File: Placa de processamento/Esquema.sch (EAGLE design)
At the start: 11 parts

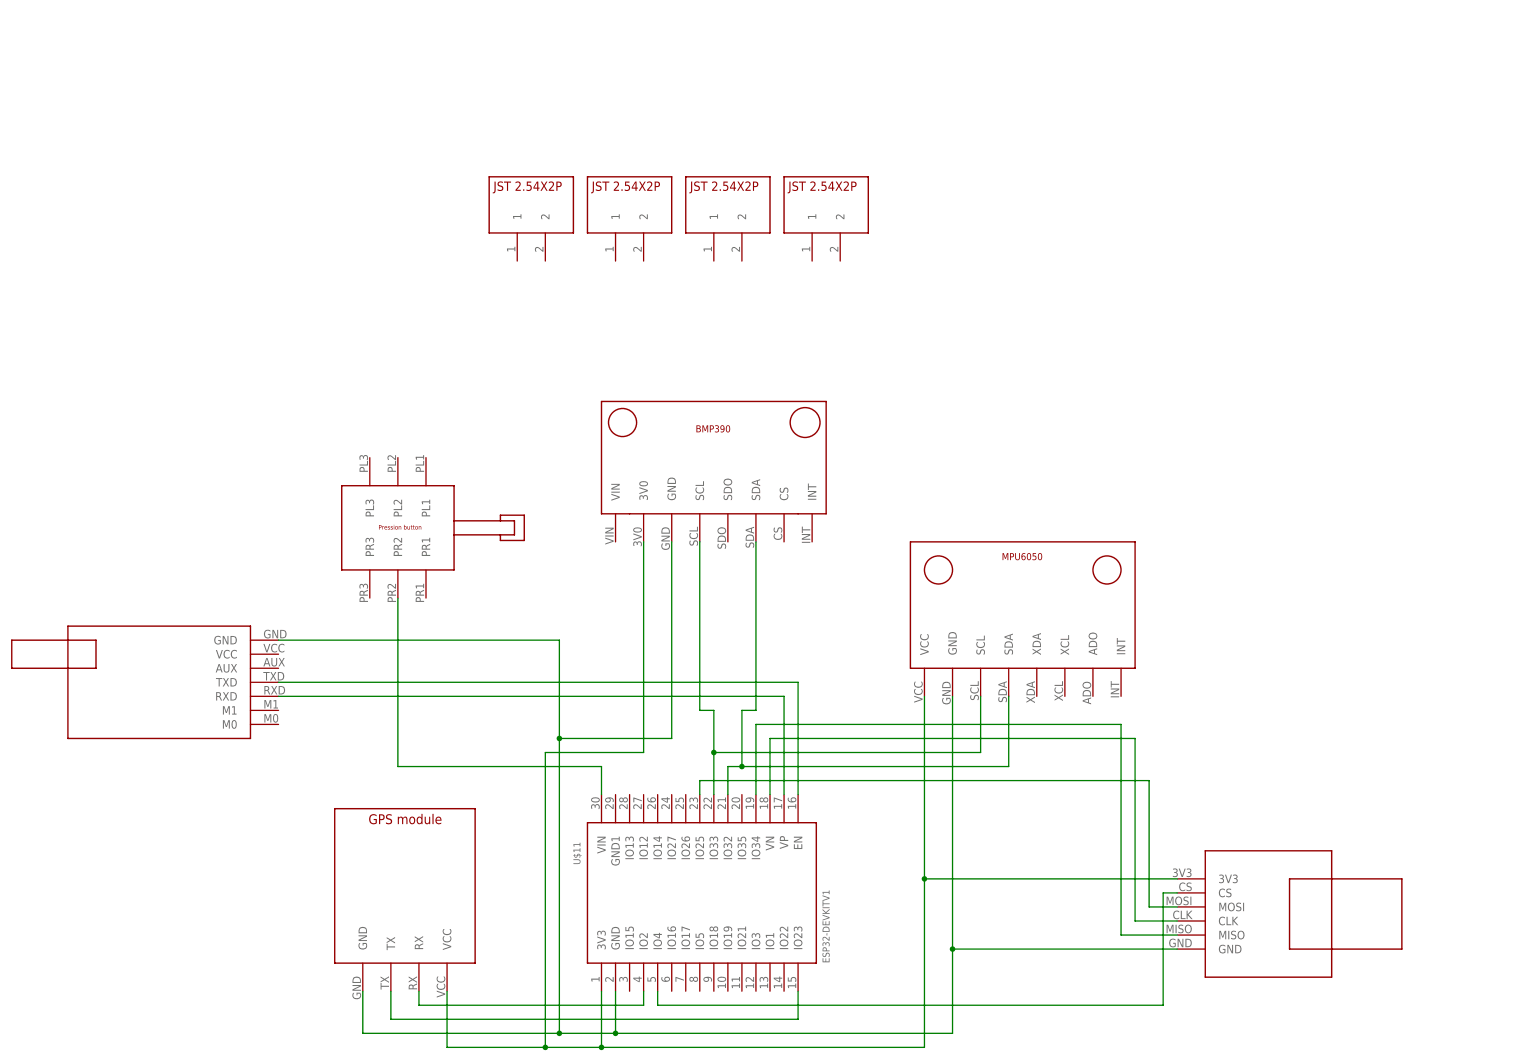
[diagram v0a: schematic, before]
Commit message: Roteamento da placa
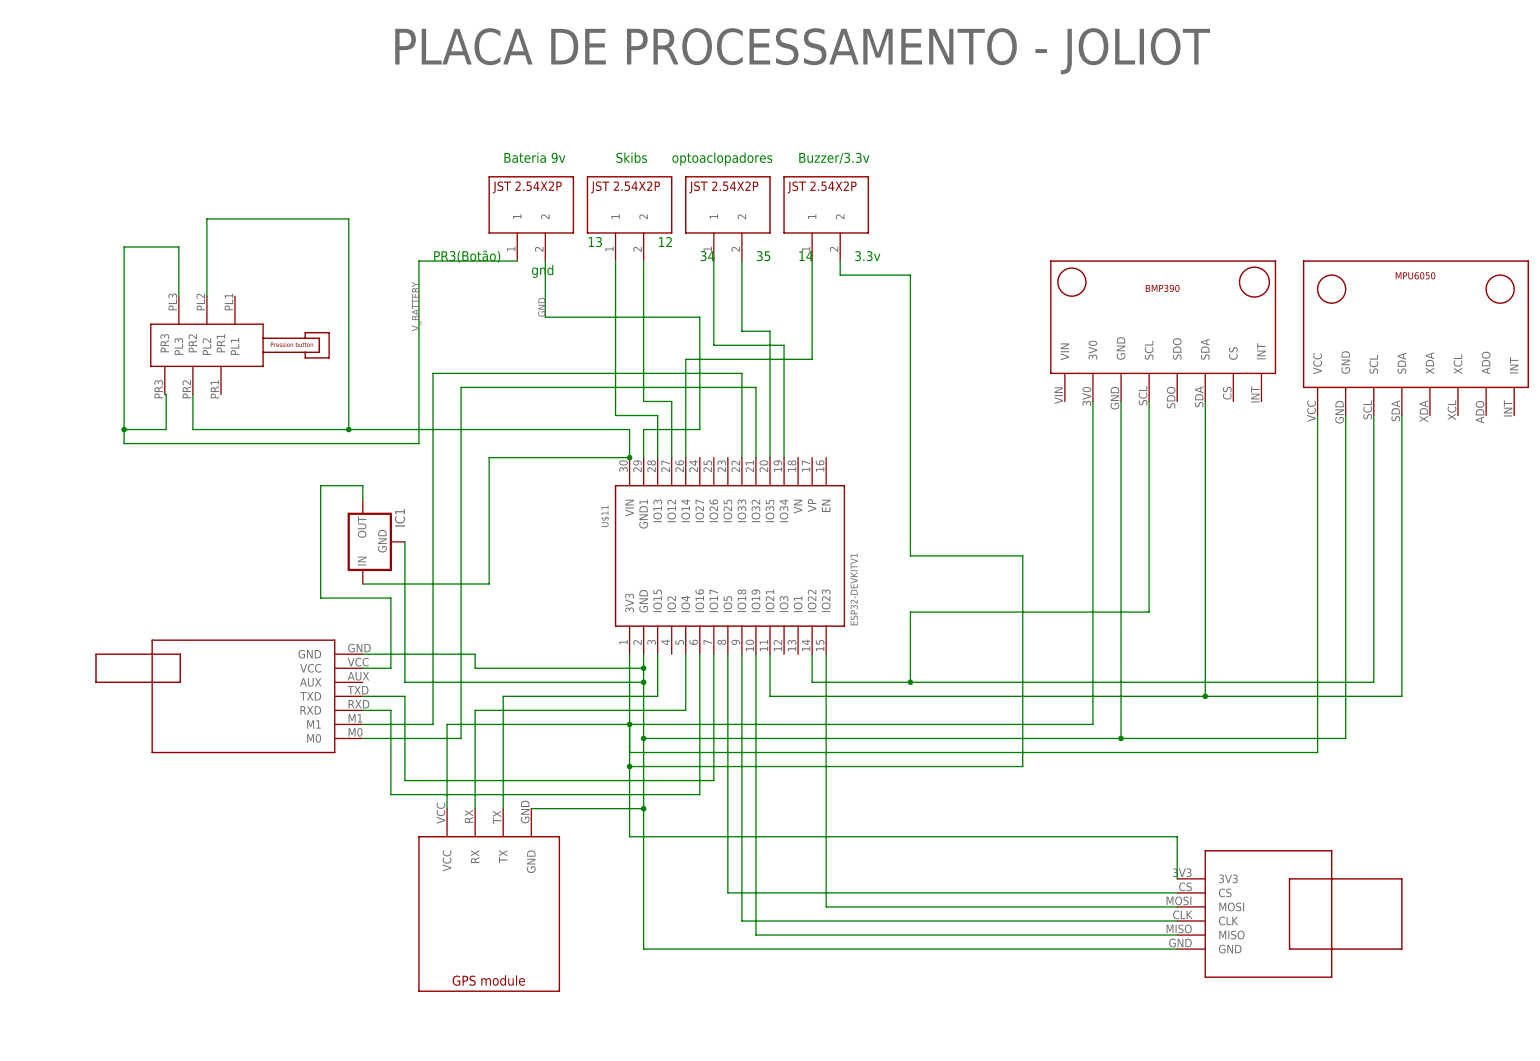
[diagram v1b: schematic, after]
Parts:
- added IC1: (no value), v-reg:78LXX
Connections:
- new net GND: U$11.GND1, U$7.2
- new net N$12: IC1.OUT, U$2.VCC
- new net N$15: U$11.IO18, U$8.CLK
- new net N$16: U$11.IO19, U$8.MISO
- new net N$19: U$11.IO13, U$6.1
- new net N$20: U$11.IO12, U$6.2
- new net N$21: U$11.IO14, U$4.1
- new net N$22: U$11.IO34, U$5.1
- new net N$23: U$11.IO35, U$5.2
- new net V_BATTERY: U$10.PL3, U$10.PR3, U$7.1
- net N$1: now also U$11.IO21; no longer U$11.IO32
- net N$10: now also U$11.IO33, U$2.M1; no longer U$11.IO34, U$8.MISO
- net N$11: now also U$11.IO32, U$2.M0; no longer U$10.PR2, U$11.VIN
- net N$13: now also U$11.IO5, U$8.CS; no longer U$11.VP, U$2.RXD
- net N$14: now also U$11.IO23, U$8.MOSI; no longer U$11.EN, U$2.TXD
- net N$2: now also U$11.IO22; no longer U$11.IO33
- net N$3: now also U$4.2
- net N$4: now also IC1.GND
- net N$5: now also U$11.IO4, U$3.RX; no longer U$11.IO23, U$3.TX
- net N$6: now also U$11.IO15, U$3.TX; no longer U$11.IO2, U$3.RX
- net N$7: now also IC1.IN, U$10.PL2, U$10.PR2, U$11.VIN; no longer U$11.IO4, U$8.CS
- net N$8: now also U$11.IO17, U$2.TXD; no longer U$11.IO25, U$8.MOSI
- net N$9: now also U$11.IO16, U$2.RXD; no longer U$11.VN, U$8.CLK
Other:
- note added: "12"
- note added: "13"
- note added: "14"
- note added: "3.3v"
- note added: "34"
- note added: "35"
- note added: "Bateria 9v"
- note added: "Buzzer/3.3v"
- note added: "PLACA DE PROCESSAMENTO - JOLIOT"
- note added: "PR3(Botão)"
- note added: "Skibs"
- note added: "gnd"
- note added: "optoaclopadores"
- moved on the sheet: U$11

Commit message: Update
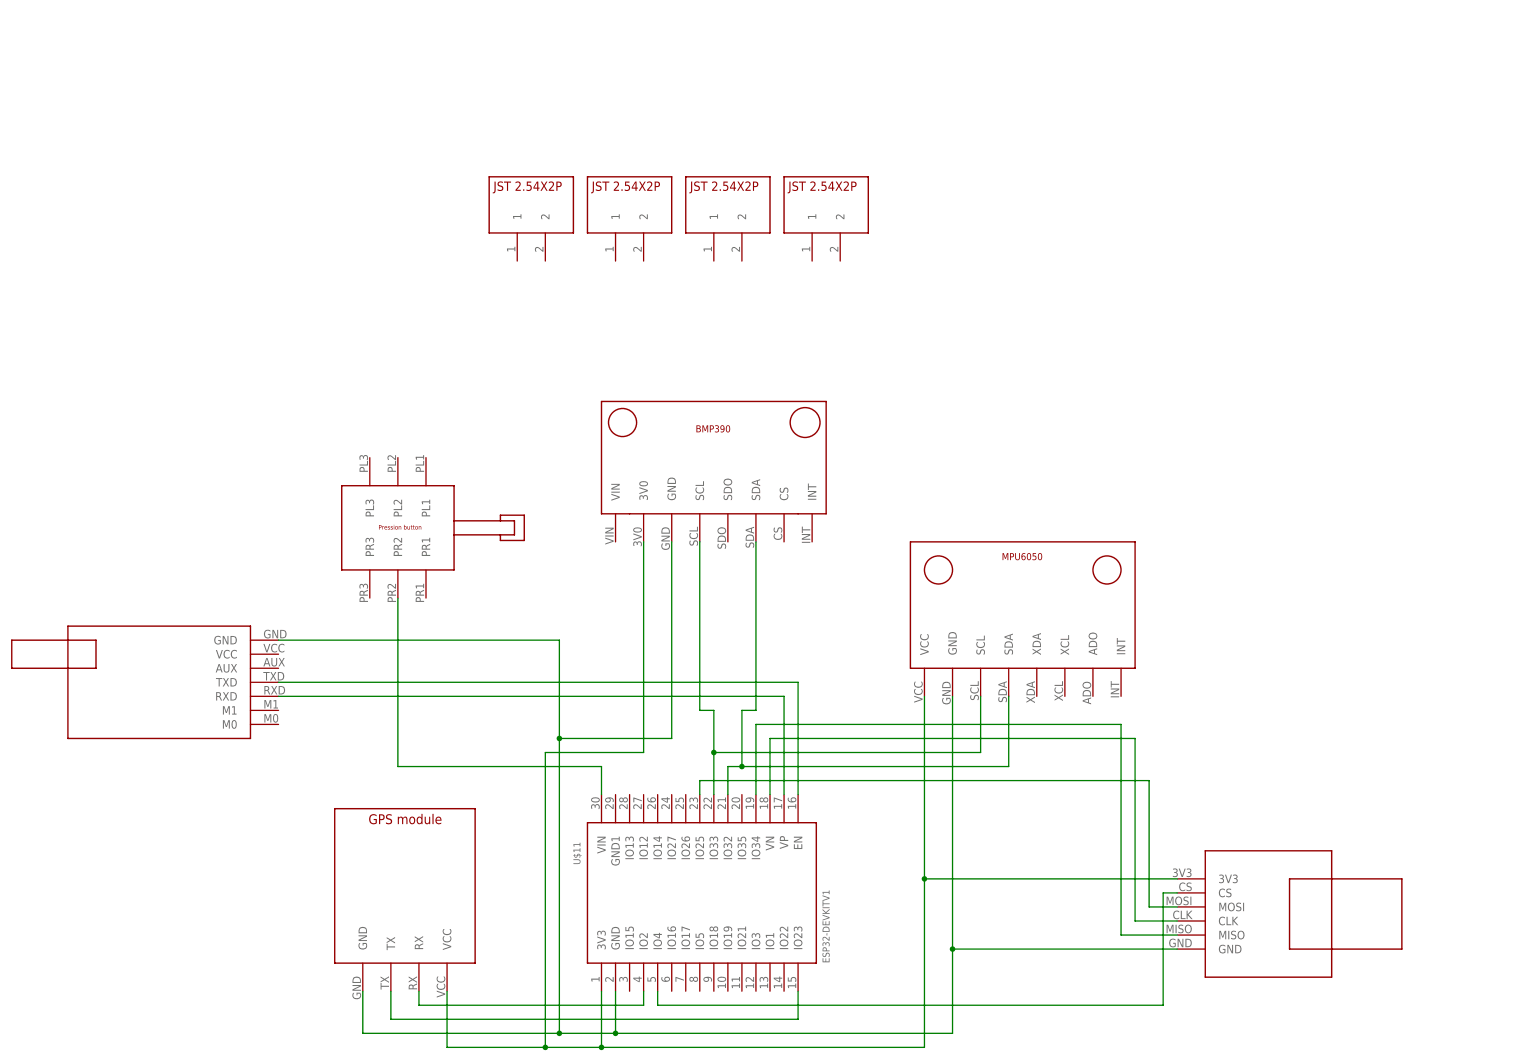
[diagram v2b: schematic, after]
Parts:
- removed IC1: (no value), v-reg:78LXX
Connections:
- removed net GND: U$11.GND1, U$7.2
- removed net N$12: IC1.OUT, U$2.VCC
- removed net N$15: U$11.IO18, U$8.CLK
- removed net N$16: U$11.IO19, U$8.MISO
- removed net N$19: U$11.IO13, U$6.1
- removed net N$20: U$11.IO12, U$6.2
- removed net N$21: U$11.IO14, U$4.1
- removed net N$22: U$11.IO34, U$5.1
- removed net N$23: U$11.IO35, U$5.2
- removed net V_BATTERY: U$10.PL3, U$10.PR3, U$7.1
- net N$1: now also U$11.IO32; no longer U$11.IO21
- net N$10: now also U$11.IO34, U$8.MISO; no longer U$11.IO33, U$2.M1
- net N$11: now also U$10.PR2, U$11.VIN; no longer U$11.IO32, U$2.M0
- net N$13: now also U$11.VP, U$2.RXD; no longer U$11.IO5, U$8.CS
- net N$14: now also U$11.EN, U$2.TXD; no longer U$11.IO23, U$8.MOSI
- net N$2: now also U$11.IO33; no longer U$11.IO22
- net N$3: no longer U$4.2
- net N$4: no longer IC1.GND
- net N$5: now also U$11.IO23, U$3.TX; no longer U$11.IO4, U$3.RX
- net N$6: now also U$11.IO2, U$3.RX; no longer U$11.IO15, U$3.TX
- net N$7: now also U$11.IO4, U$8.CS; no longer IC1.IN, U$10.PL2, U$10.PR2, U$11.VIN
- net N$8: now also U$11.IO25, U$8.MOSI; no longer U$11.IO17, U$2.TXD
- net N$9: now also U$11.VN, U$8.CLK; no longer U$11.IO16, U$2.RXD
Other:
- note removed: "12"
- note removed: "13"
- note removed: "14"
- note removed: "3.3v"
- note removed: "34"
- note removed: "35"
- note removed: "Bateria 9v"
- note removed: "Buzzer/3.3v"
- note removed: "PLACA DE PROCESSAMENTO - JOLIOT"
- note removed: "PR3(Botão)"
- note removed: "Skibs"
- note removed: "gnd"
- note removed: "optoaclopadores"
- moved on the sheet: U$11
